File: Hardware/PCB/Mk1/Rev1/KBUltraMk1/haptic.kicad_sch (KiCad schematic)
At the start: 8 parts, among them M101 Motor_DC_ALT, M102 Motor_DC_ALT, M103 Motor_DC_ALT, M104 Motor_DC_ALT, U101 DRV2605LDGS, U104 DRV2605LDGS, U105 DRV2605LDGS, U106 DRV2605LDGS

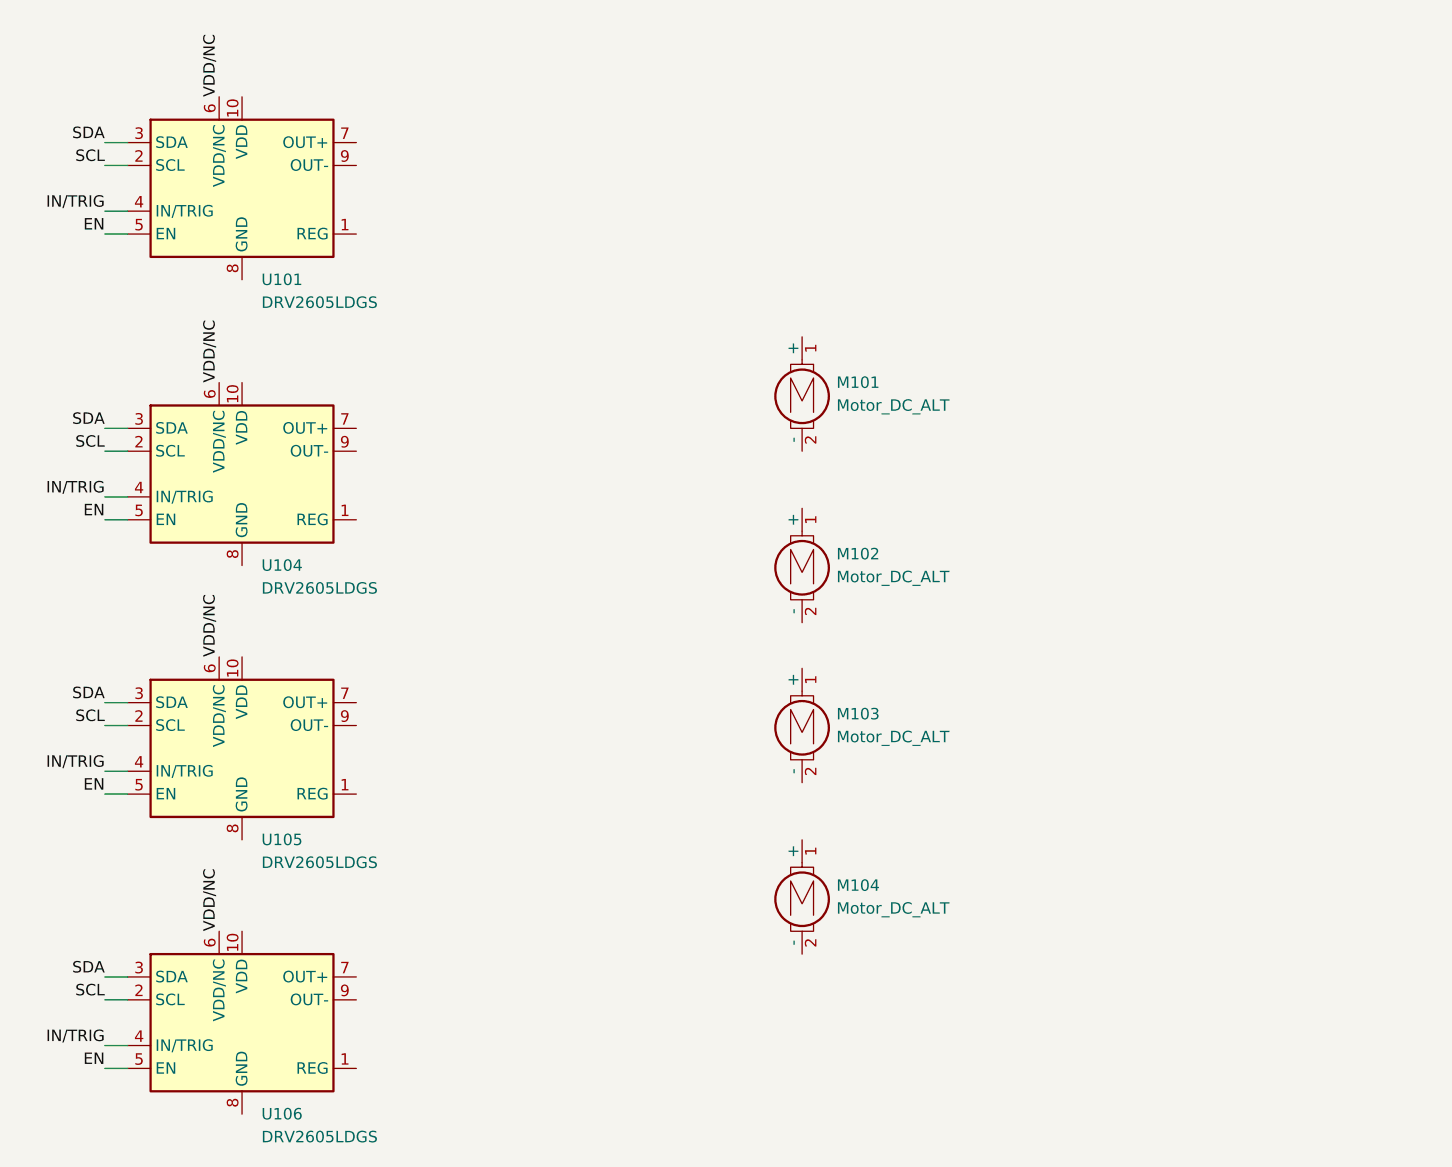
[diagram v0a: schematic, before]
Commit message: A
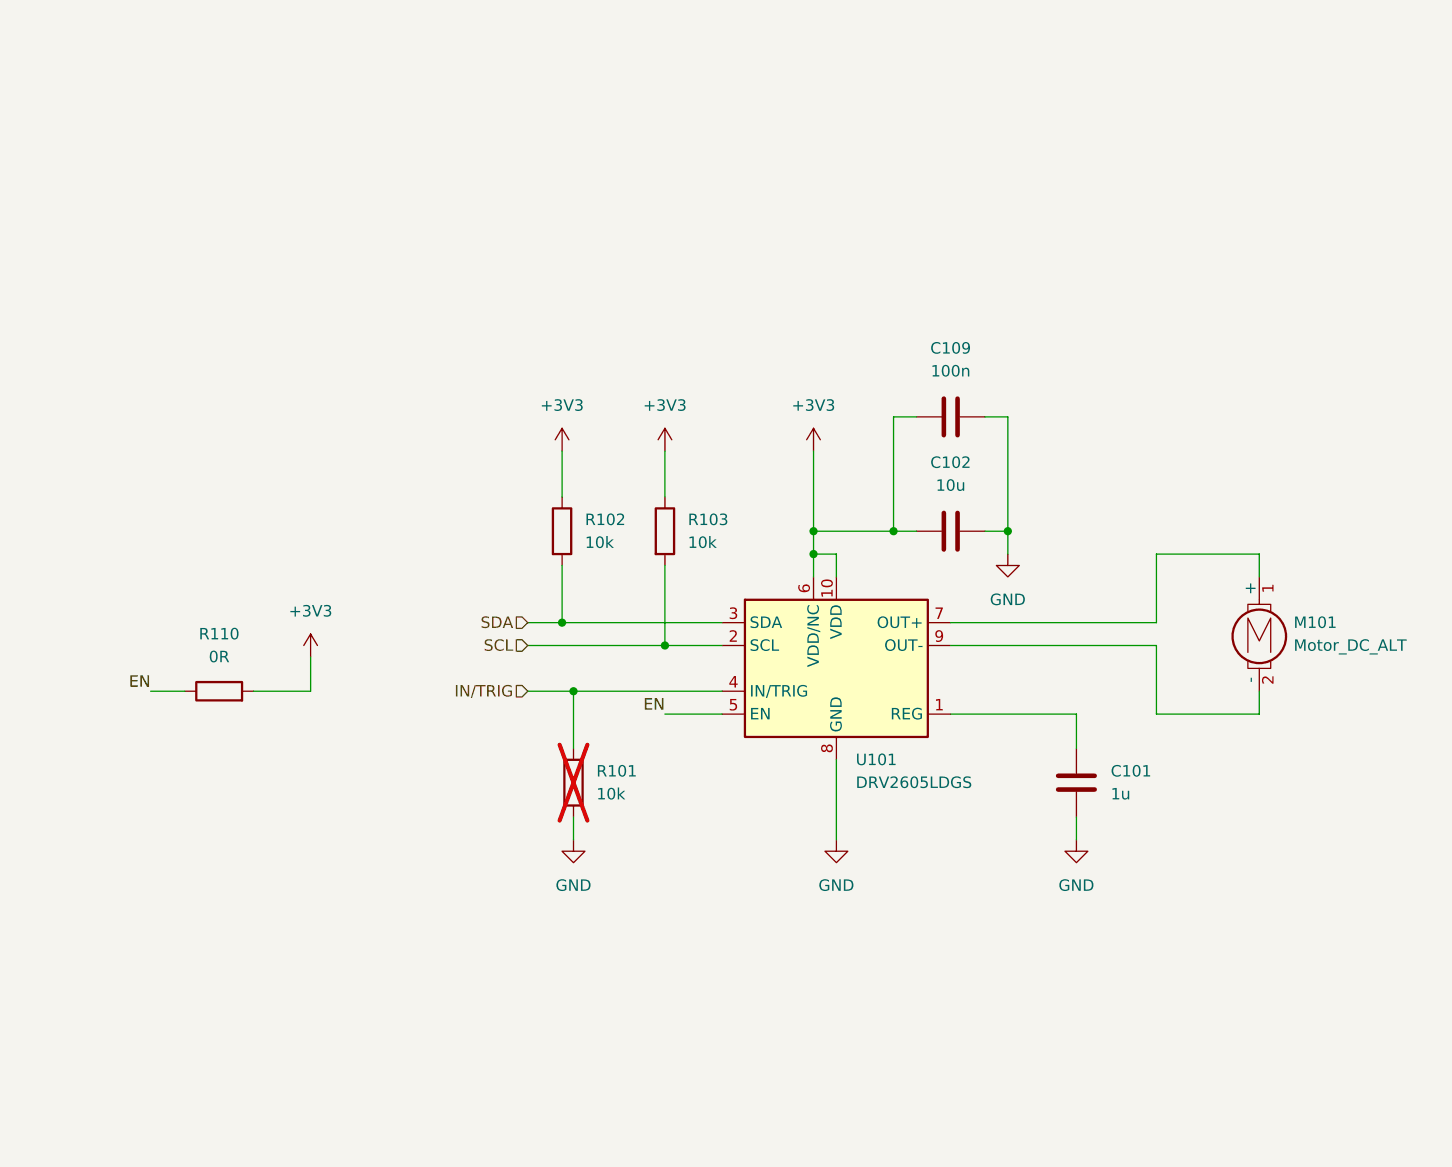
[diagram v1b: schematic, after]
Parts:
- removed M102, M103, M104: Motor_DC_ALT, symbol Motor:Motor_DC_ALT
- removed U104, U105, U106: DRV2605LDGS, Package_SO:TSSOP-10_3x3mm_P0.5mm, symbol Driver:DRV2605LDGS
- added C101: 1u, Capacitor_SMD:C_0603_1608Metric, symbol Device:C
- added C102: 10u, Capacitor_SMD:C_0805_2012Metric, symbol Device:C
- added C109: 100n, Capacitor_SMD:C_0402_1005Metric, symbol Device:C
- added R101, R102, R103: 10k, Resistor_SMD:R_0603_1608Metric, symbol Device:R
- added R110: 0R, Resistor_SMD:R_0603_1608Metric, symbol Device:R
- M101: footprint (none) -> Connector_PinHeader_2.54mm:PinHeader_1x02_P2.54mm_Vertical
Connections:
- net VDD/NC is gone; now on net +3V3: U101.6 (VDD/NC)
- net EN: now also R110.1
- net SCL: now also R103.2
- net SDA: now also R102.2
- net at U101.1 (REG): now also C101.1
- net +3V3: now reaches U101.10 (VDD)
- net +3V3: now also C102.1, C109.1, R102.1, R103.1, R110.2
- net at U101.7 (OUT+): now also M101.1 (+)
- net GND: now reaches U101.8 (GND)
- net GND: now also C101.2, C102.2, C109.2, R101.2
- net at U101.9 (OUT-): now also M101.2 (-)
- net IN/TRIG renamed IN/TRIG
- net IN/TRIG: now also R101.1
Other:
- moved on the sheet: M101, U101
